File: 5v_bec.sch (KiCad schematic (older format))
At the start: 9 parts, among them U4 LM2677S-5.0

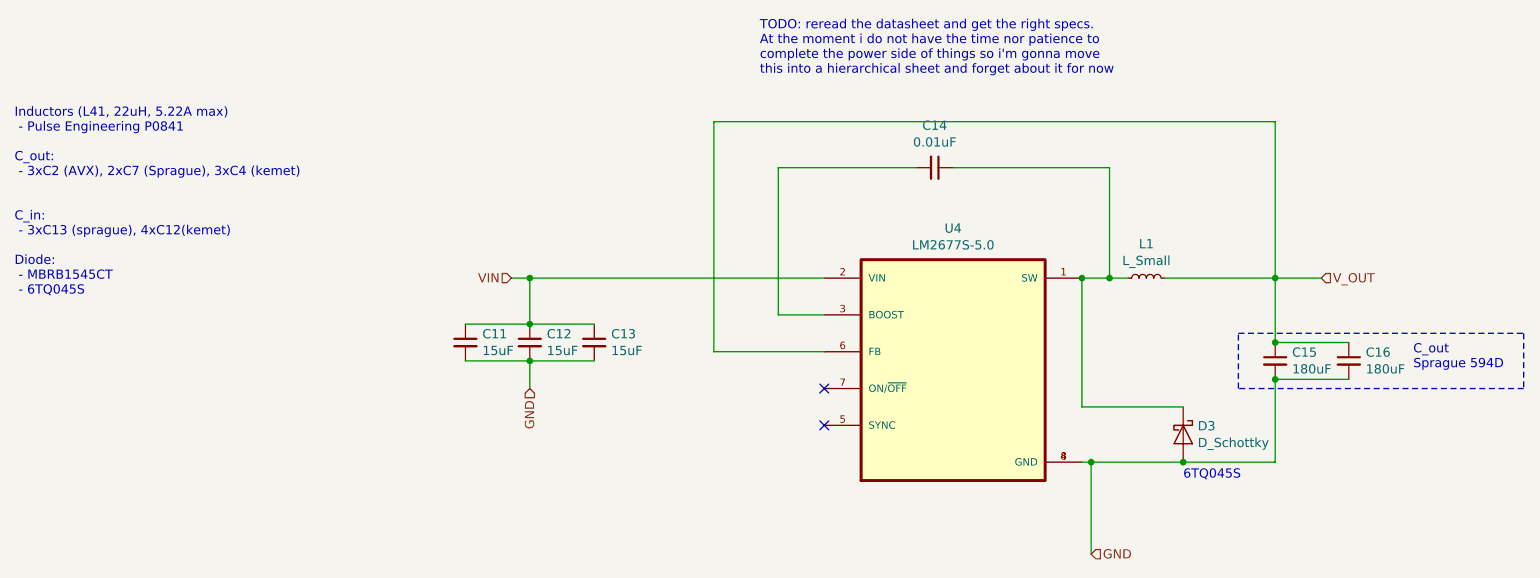
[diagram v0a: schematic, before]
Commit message: no longer a hat lol
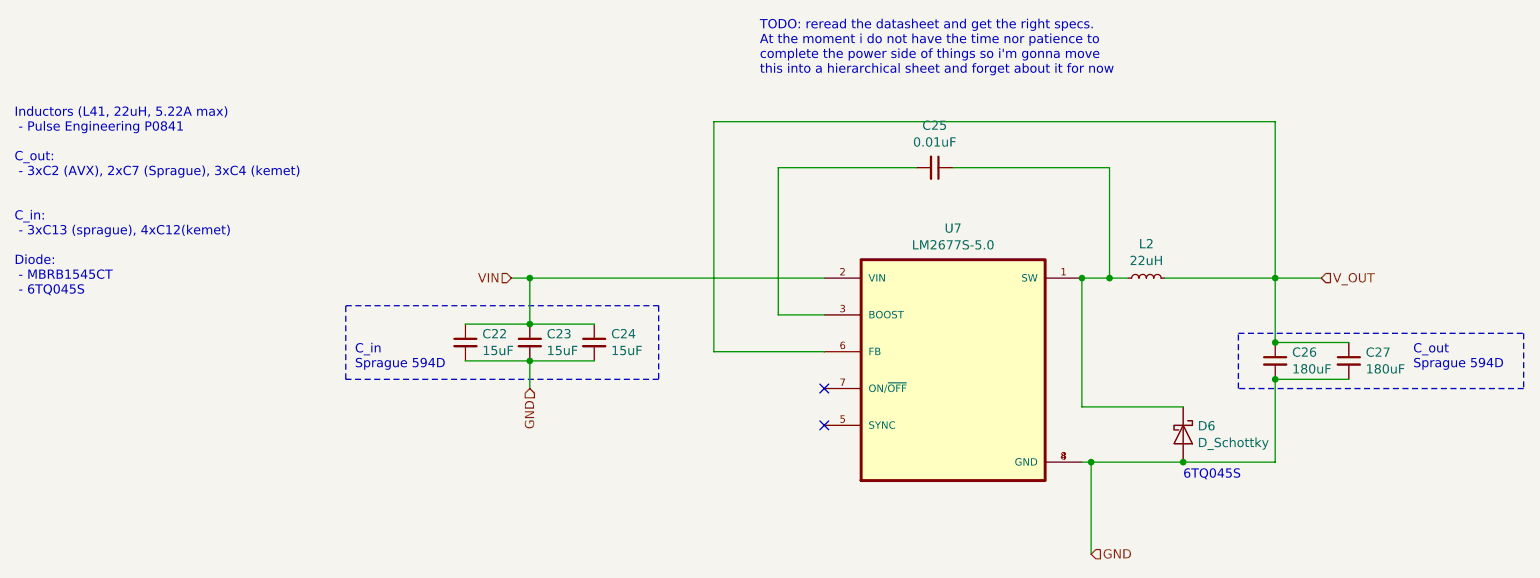
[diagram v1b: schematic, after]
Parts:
- C11, C12, C13: footprint (none) -> Capacitor_Tantalum_SMD:CP_EIA-7260-15_AVX-R_Pad2.68x6.30mm_HandSolder
- C14: footprint (none) -> Capacitor_SMD:C_0805_2012Metric_Pad1.15x1.40mm_HandSolder
- C15, C16: footprint (none) -> Capacitor_Tantalum_SMD:CP_EIA-7260-38_AVX-R_Pad2.68x6.30mm_HandSolder
- D3: footprint (none) -> TO254P1521X483-4N:TO254P1521X483-4N
- L1: value L_Small -> 22uH; footprint (none) -> Inductor_SMD:L_10.4x10.4_H4.8
- U4: footprint TO127P1435X464-8N -> LM2677S-5:TO127P1435X464-8N
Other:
- note added: "C_in\nSprague 594D"
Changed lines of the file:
@@
 $Descr A4 11693 8268
 encoding utf-8
-Sheet 4 8
+Sheet 7 8
 Title ""
 Date ""
@@
 AR Path="/619C4F1E/6175201D" Ref="U7"  Part="1"
 AR Path="/619C86ED/6175201D" Ref="U?"  Part="1"
-F 0 "U4" H 6000 5020 50  0000 C CNN
+F 0 "U7" H 6000 5020 50  0000 C CNN
 F 1 "LM2677S-5.0" H 6000 4929 50  0000 C CNN
-F 2 "TO127P1435X464-8N" H 6000 4250 50  0001 L BNN
+F 2 "LM2677S-5:TO127P1435X464-8N" H 6000 4250 50  0001 L BNN
 F 3 "" H 6000 4250 50  0001 L BNN
 	1    6000 4250
@@
 AR Path="/619C4F1E/617603E2" Ref="D6"  Part="1"
 AR Path="/619C86ED/617603E2" Ref="D?"  Part="1"
-F 0 "D3" V 7204 4679 50  0000 L CNN
+F 0 "D6" V 7204 4679 50  0000 L CNN
 F 1 "D_Schottky" V 7295 4679 50  0000 L CNN
-F 2 "" H 7250 4600 50  0001 C CNN
+F 2 "TO254P1521X483-4N:TO254P1521X483-4N" H 7250 4600 50  0001 C CNN
 F 3 "~" H 7250 4600 50  0001 C CNN
 	1    7250 4600
@@
 AR Path="/619C4F1E/61768ED3" Ref="L2"  Part="1"
 AR Path="/619C86ED/61768ED3" Ref="L?"  Part="1"
-F 0 "L1" V 7235 3750 50  0000 C CNN
-F 1 "L_Small" V 7144 3750 50  0000 C CNN
-F 2 "" H 7050 3750 50  0001 C CNN
+F 0 "L2" V 7235 3750 50  0000 C CNN
+F 1 "22uH" V 7144 3750 50  0000 C CNN
+F 2 "Inductor_SMD:L_10.4x10.4_H4.8" H 7050 3750 50  0001 C CNN
 F 3 "~" H 7050 3750 50  0001 C CNN
 	1    7050 3750
@@
 AR Path="/619C4F1E/6176CADF" Ref="C25"  Part="1"
 AR Path="/619C86ED/6176CADF" Ref="C?"  Part="1"
-F 0 "C14" V 5671 3150 50  0000 C CNN
+F 0 "C25" V 5671 3150 50  0000 C CNN
 F 1 "0.01uF" V 5762 3150 50  0000 C CNN
-F 2 "" H 5900 3150 50  0001 C CNN
+F 2 "Capacitor_SMD:C_0805_2012Metric_Pad1.15x1.40mm_HandSolder" H 5900 3150 50  0001 C CNN
 F 3 "~" H 5900 3150 50  0001 C CNN
 	1    5900 3150
@@
 AR Path="/6175047F/61A51E59" Ref="C15"  Part="1"
 AR Path="/619C4F1E/61A51E59" Ref="C26"  Part="1"
-F 0 "C15" H 7842 4246 50  0000 L CNN
+F 0 "C26" H 7842 4246 50  0000 L CNN
 F 1 "180uF" H 7842 4155 50  0000 L CNN
-F 2 "" H 7750 4200 50  0001 C CNN
+F 2 "Capacitor_Tantalum_SMD:CP_EIA-7260-38_AVX-R_Pad2.68x6.30mm_HandSolder" H 7750 4200 50  0001 C CNN
 F 3 "~" H 7750 4200 50  0001 C CNN
 	1    7750 4200
@@
 AR Path="/6175047F/61A52F3A" Ref="C16"  Part="1"
 AR Path="/619C4F1E/61A52F3A" Ref="C27"  Part="1"
-F 0 "C16" H 8242 4246 50  0000 L CNN
+F 0 "C27" H 8242 4246 50  0000 L CNN
 F 1 "180uF" H 8242 4155 50  0000 L CNN
-F 2 "" H 8150 4200 50  0001 C CNN
+F 2 "Capacitor_Tantalum_SMD:CP_EIA-7260-38_AVX-R_Pad2.68x6.30mm_HandSolder" H 8150 4200 50  0001 C CNN
 F 3 "~" H 8150 4200 50  0001 C CNN
 	1    8150 4200
@@
 AR Path="/6175047F/61A5F9C8" Ref="C11"  Part="1"
 AR Path="/619C4F1E/61A5F9C8" Ref="C22"  Part="1"
-F 0 "C11" H 3442 4146 50  0000 L CNN
+F 0 "C22" H 3442 4146 50  0000 L CNN
 F 1 "15uF" H 3442 4055 50  0000 L CNN
-F 2 "" H 3350 4100 50  0001 C CNN
+F 2 "Capacitor_Tantalum_SMD:CP_EIA-7260-15_AVX-R_Pad2.68x6.30mm_HandSolder" H 3350 4100 50  0001 C CNN
 F 3 "~" H 3350 4100 50  0001 C CNN
 	1    3350 4100
@@
 AR Path="/6175047F/61A60CAD" Ref="C12"  Part="1"
 AR Path="/619C4F1E/61A60CAD" Ref="C23"  Part="1"
-F 0 "C12" H 3792 4146 50  0000 L CNN
+F 0 "C23" H 3792 4146 50  0000 L CNN
 F 1 "15uF" H 3792 4055 50  0000 L CNN
-F 2 "" H 3700 4100 50  0001 C CNN
+F 2 "Capacitor_Tantalum_SMD:CP_EIA-7260-15_AVX-R_Pad2.68x6.30mm_HandSolder" H 3700 4100 50  0001 C CNN
 F 3 "~" H 3700 4100 50  0001 C CNN
 	1    3700 4100
@@
 AR Path="/6175047F/61A62459" Ref="C13"  Part="1"
 AR Path="/619C4F1E/61A62459" Ref="C24"  Part="1"
-F 0 "C13" H 4142 4146 50  0000 L CNN
+F 0 "C24" H 4142 4146 50  0000 L CNN
 F 1 "15uF" H 4142 4055 50  0000 L CNN
-F 2 "" H 4050 4100 50  0001 C CNN
+F 2 "Capacitor_Tantalum_SMD:CP_EIA-7260-15_AVX-R_Pad2.68x6.30mm_HandSolder" H 4050 4100 50  0001 C CNN
 F 3 "~" H 4050 4100 50  0001 C CNN
 	1    4050 4100
@@
 Text Notes 7250 4850 0    50   ~ 0
 6TQ045S
+Wire Notes Line
+	4400 4300 2700 4300
+Wire Notes Line
+	2700 4300 2700 3900
+Wire Notes Line
+	2700 3900 4400 3900
+Wire Notes Line
+	4400 3900 4400 4300
+Text Notes 2750 4250 0    50   ~ 0
+C_in\nSprague 594D
 $EndSCHEMATC

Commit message: power supply overhaul
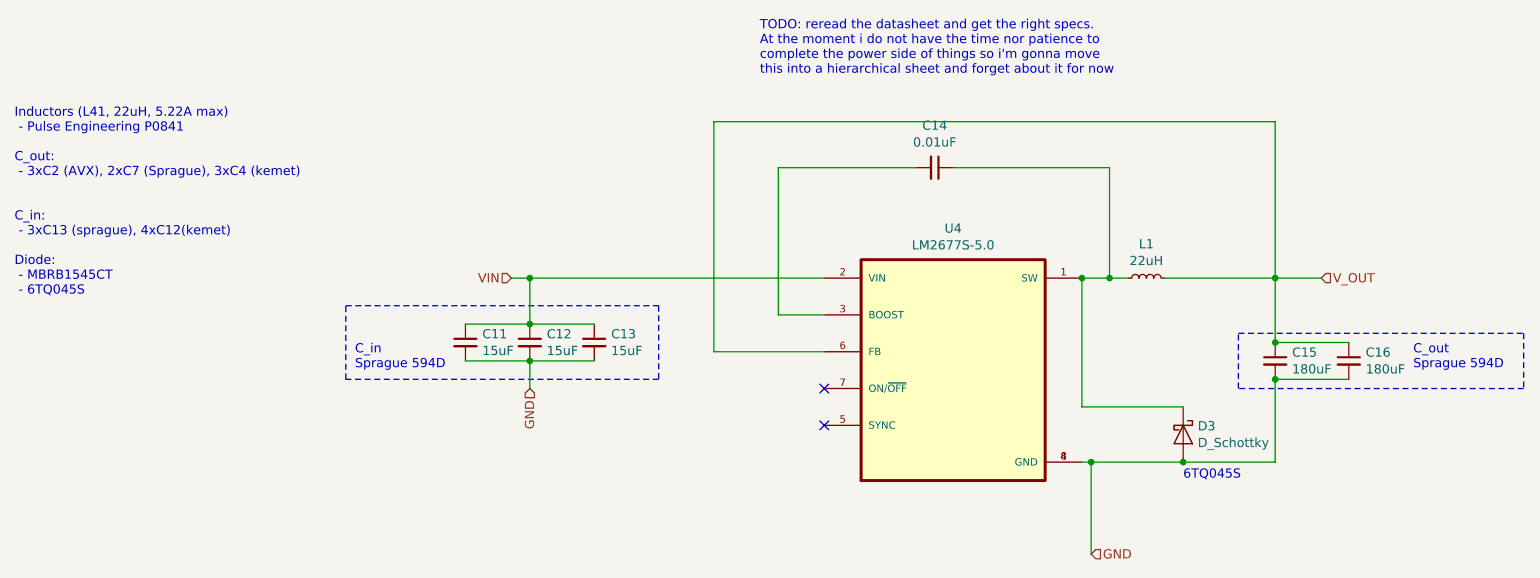
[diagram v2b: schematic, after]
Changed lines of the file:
@@
 $Descr A4 11693 8268
 encoding utf-8
-Sheet 7 8
+Sheet 7 10
 Title ""
 Date ""
@@
 AR Path="/619C4F1E/6175201D" Ref="U7"  Part="1"
 AR Path="/619C86ED/6175201D" Ref="U?"  Part="1"
-F 0 "U7" H 6000 5020 50  0000 C CNN
+F 0 "U4" H 6000 5020 50  0000 C CNN
 F 1 "LM2677S-5.0" H 6000 4929 50  0000 C CNN
 F 2 "LM2677S-5:TO127P1435X464-8N" H 6000 4250 50  0001 L BNN
@@
 AR Path="/619C4F1E/617603E2" Ref="D6"  Part="1"
 AR Path="/619C86ED/617603E2" Ref="D?"  Part="1"
-F 0 "D6" V 7204 4679 50  0000 L CNN
+F 0 "D3" V 7204 4679 50  0000 L CNN
 F 1 "D_Schottky" V 7295 4679 50  0000 L CNN
 F 2 "TO254P1521X483-4N:TO254P1521X483-4N" H 7250 4600 50  0001 C CNN
@@
 AR Path="/619C4F1E/61768ED3" Ref="L2"  Part="1"
 AR Path="/619C86ED/61768ED3" Ref="L?"  Part="1"
-F 0 "L2" V 7235 3750 50  0000 C CNN
+F 0 "L1" V 7235 3750 50  0000 C CNN
 F 1 "22uH" V 7144 3750 50  0000 C CNN
 F 2 "Inductor_SMD:L_10.4x10.4_H4.8" H 7050 3750 50  0001 C CNN
@@
 AR Path="/619C4F1E/6176CADF" Ref="C25"  Part="1"
 AR Path="/619C86ED/6176CADF" Ref="C?"  Part="1"
-F 0 "C25" V 5671 3150 50  0000 C CNN
+F 0 "C14" V 5671 3150 50  0000 C CNN
 F 1 "0.01uF" V 5762 3150 50  0000 C CNN
 F 2 "Capacitor_SMD:C_0805_2012Metric_Pad1.15x1.40mm_HandSolder" H 5900 3150 50  0001 C CNN
@@
 AR Path="/6175047F/61A51E59" Ref="C15"  Part="1"
 AR Path="/619C4F1E/61A51E59" Ref="C26"  Part="1"
-F 0 "C26" H 7842 4246 50  0000 L CNN
+F 0 "C15" H 7842 4246 50  0000 L CNN
 F 1 "180uF" H 7842 4155 50  0000 L CNN
 F 2 "Capacitor_Tantalum_SMD:CP_EIA-7260-38_AVX-R_Pad2.68x6.30mm_HandSolder" H 7750 4200 50  0001 C CNN
@@
 AR Path="/6175047F/61A52F3A" Ref="C16"  Part="1"
 AR Path="/619C4F1E/61A52F3A" Ref="C27"  Part="1"
-F 0 "C27" H 8242 4246 50  0000 L CNN
+F 0 "C16" H 8242 4246 50  0000 L CNN
 F 1 "180uF" H 8242 4155 50  0000 L CNN
 F 2 "Capacitor_Tantalum_SMD:CP_EIA-7260-38_AVX-R_Pad2.68x6.30mm_HandSolder" H 8150 4200 50  0001 C CNN
@@
 AR Path="/6175047F/61A5F9C8" Ref="C11"  Part="1"
 AR Path="/619C4F1E/61A5F9C8" Ref="C22"  Part="1"
-F 0 "C22" H 3442 4146 50  0000 L CNN
+F 0 "C11" H 3442 4146 50  0000 L CNN
 F 1 "15uF" H 3442 4055 50  0000 L CNN
 F 2 "Capacitor_Tantalum_SMD:CP_EIA-7260-15_AVX-R_Pad2.68x6.30mm_HandSolder" H 3350 4100 50  0001 C CNN
@@
 AR Path="/6175047F/61A60CAD" Ref="C12"  Part="1"
 AR Path="/619C4F1E/61A60CAD" Ref="C23"  Part="1"
-F 0 "C23" H 3792 4146 50  0000 L CNN
+F 0 "C12" H 3792 4146 50  0000 L CNN
 F 1 "15uF" H 3792 4055 50  0000 L CNN
 F 2 "Capacitor_Tantalum_SMD:CP_EIA-7260-15_AVX-R_Pad2.68x6.30mm_HandSolder" H 3700 4100 50  0001 C CNN
@@
 AR Path="/6175047F/61A62459" Ref="C13"  Part="1"
 AR Path="/619C4F1E/61A62459" Ref="C24"  Part="1"
-F 0 "C24" H 4142 4146 50  0000 L CNN
+F 0 "C13" H 4142 4146 50  0000 L CNN
 F 1 "15uF" H 4142 4055 50  0000 L CNN
 F 2 "Capacitor_Tantalum_SMD:CP_EIA-7260-15_AVX-R_Pad2.68x6.30mm_HandSolder" H 4050 4100 50  0001 C CNN
